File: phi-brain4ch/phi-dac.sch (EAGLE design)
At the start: 146 parts, among them IC1 PCM1792A, IC10 LM317, IC11 LM337, IC2 OPA1632D, IC3 OPA1632D, IC4 OPA1632D, IC6 OPA1632D, IC7 REG1117-5, IC8 ADP3301ARZ-3.3, IC9 MGJ2D121515SC, J1 CUI-RCJ-2123, J5 DC21P

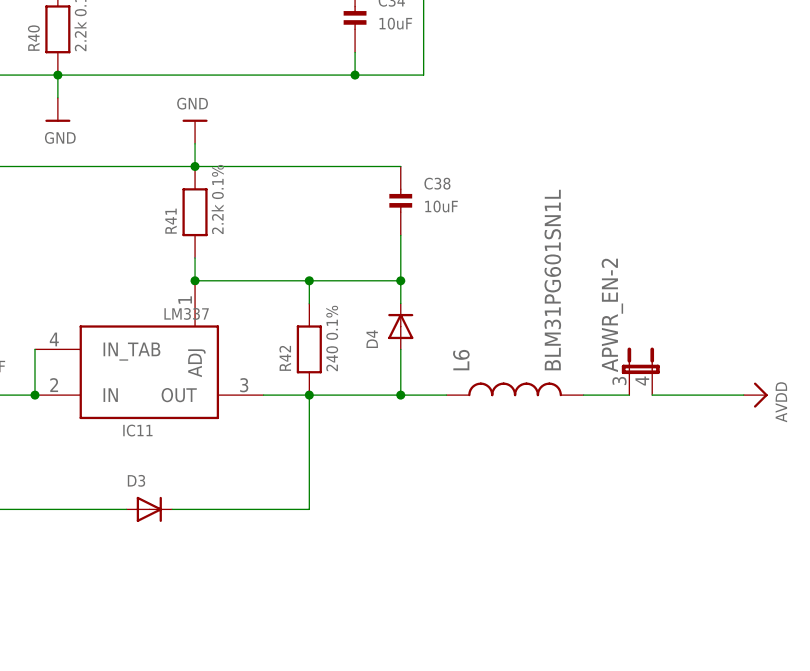
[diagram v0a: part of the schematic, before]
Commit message: wip
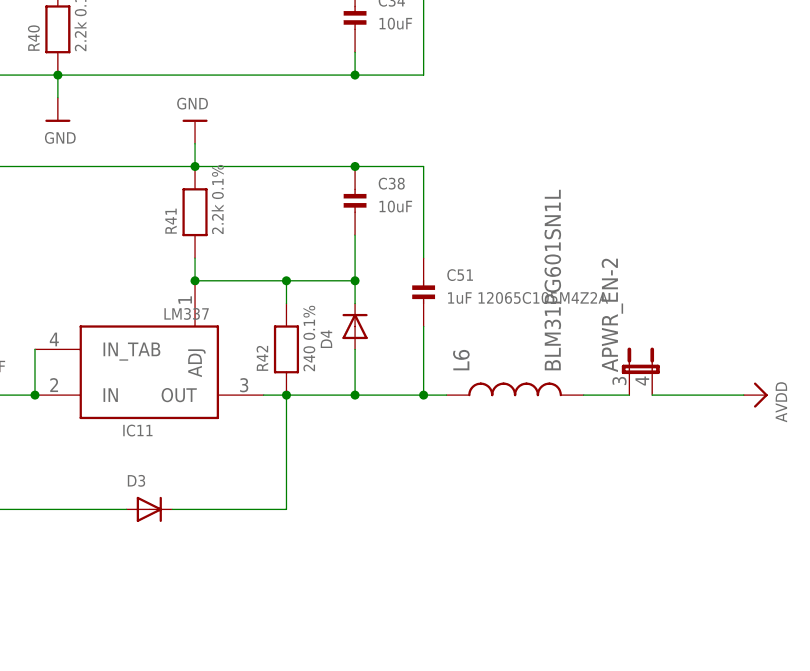
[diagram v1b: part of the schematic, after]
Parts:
- added C51: 1uF 12065C105M4Z2A, microbuilder:CAP_CERAMIC1206
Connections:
- net GND: now also C51.P$1
- net N$57: now also C51.P$2
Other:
- moved on the sheet: C38, D4, R42
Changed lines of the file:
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@@
 <part name="C49" library="microbuilder" deviceset="CAP_CERAMIC" device="0603" value="0.1u"/>
 <part name="C50" library="microbuilder" deviceset="CAP_CERAMIC" device="0603" value="0.1u"/>
+<part name="C51" library="microbuilder" deviceset="CAP_CERAMIC" device="1206" value="1uF 12065C105M4Z2A"/>
 </parts>
 <sheets>
@@
 <instance part="C37" gate="G$1" x="190.5" y="147.32"/>
 <instance part="R41" gate="G$1" x="218.44" y="165.1" rot="R90"/>
-<instance part="R42" gate="G$1" x="231.14" y="149.86" rot="R90"/>
+<instance part="R42" gate="G$1" x="228.6" y="149.86" rot="R90"/>
 <instance part="U$29" gate="G$1" x="218.44" y="175.26" rot="R180"/>
-<instance part="C38" gate="G$1" x="241.3" y="165.1"/>
-<instance part="D4" gate="G$1" x="241.3" y="152.4" rot="R90"/>
+<instance part="C38" gate="G$1" x="236.22" y="165.1"/>
+<instance part="D4" gate="G$1" x="236.22" y="152.4" rot="R90"/>
 <instance part="L6" gate="G$1" x="254" y="144.78" rot="R90"/>
 <instance part="U$30" gate="G$1" x="281.94" y="144.78" rot="R270"/>
@@
 <instance part="C49" gate="G$1" x="149.86" y="-22.86"/>
 <instance part="C50" gate="G$1" x="149.86" y="-12.7"/>
+<instance part="C51" gate="G$1" x="243.84" y="154.94"/>
 </instances>
 <busses>
@@
 <junction x="218.44" y="170.18"/>
 <pinref part="C38" gate="G$1" pin="P$1"/>
-<wire x1="218.44" y1="170.18" x2="241.3" y2="170.18" width="0.1524" layer="91"/>
+<wire x1="218.44" y1="170.18" x2="236.22" y2="170.18" width="0.1524" layer="91"/>
+<pinref part="C51" gate="G$1" pin="P$1"/>
+<wire x1="236.22" y1="170.18" x2="243.84" y2="170.18" width="0.1524" layer="91"/>
+<wire x1="243.84" y1="170.18" x2="243.84" y2="160.02" width="0.1524" layer="91"/>
+<junction x="236.22" y="170.18"/>
 </segment>
 <segment>
@@
 <pinref part="D3" gate="G$1" pin="C"/>
 <pinref part="R42" gate="G$1" pin="1"/>
-<wire x1="215.9" y1="132.08" x2="231.14" y2="132.08" width="0.1524" layer="91"/>
-<wire x1="231.14" y1="132.08" x2="231.14" y2="144.78" width="0.1524" layer="91"/>
+<wire x1="215.9" y1="132.08" x2="228.6" y2="132.08" width="0.1524" layer="91"/>
+<wire x1="228.6" y1="132.08" x2="228.6" y2="144.78" width="0.1524" layer="91"/>
 <pinref part="IC11" gate="G$1" pin="OUT"/>
-<wire x1="231.14" y1="144.78" x2="226.06" y2="144.78" width="0.1524" layer="91"/>
-<junction x="231.14" y="144.78"/>
-<wire x1="231.14" y1="144.78" x2="241.3" y2="144.78" width="0.1524" layer="91"/>
-<wire x1="241.3" y1="144.78" x2="241.3" y2="149.86" width="0.1524" layer="91"/>
+<wire x1="228.6" y1="144.78" x2="226.06" y2="144.78" width="0.1524" layer="91"/>
+<junction x="228.6" y="144.78"/>
+<wire x1="228.6" y1="144.78" x2="236.22" y2="144.78" width="0.1524" layer="91"/>
+<wire x1="236.22" y1="144.78" x2="236.22" y2="149.86" width="0.1524" layer="91"/>
 <pinref part="D4" gate="G$1" pin="A"/>
 <pinref part="L6" gate="G$1" pin="1"/>
-<wire x1="246.38" y1="144.78" x2="241.3" y2="144.78" width="0.1524" layer="91"/>
-<junction x="241.3" y="144.78"/>
+<wire x1="246.38" y1="144.78" x2="243.84" y2="144.78" width="0.1524" layer="91"/>
+<junction x="236.22" y="144.78"/>
+<junction x="243.84" y="144.78"/>
+<wire x1="243.84" y1="144.78" x2="236.22" y2="144.78" width="0.1524" layer="91"/>
+<pinref part="C51" gate="G$1" pin="P$2"/>
+<wire x1="243.84" y1="152.4" x2="243.84" y2="144.78" width="0.1524" layer="91"/>
 </segment>
 </net>
@@
 <wire x1="218.44" y1="157.48" x2="218.44" y2="160.02" width="0.1524" layer="91"/>
 <pinref part="R42" gate="G$1" pin="2"/>
-<wire x1="231.14" y1="154.94" x2="231.14" y2="157.48" width="0.1524" layer="91"/>
-<wire x1="231.14" y1="157.48" x2="218.44" y2="157.48" width="0.1524" layer="91"/>
+<wire x1="228.6" y1="154.94" x2="228.6" y2="157.48" width="0.1524" layer="91"/>
+<wire x1="228.6" y1="157.48" x2="218.44" y2="157.48" width="0.1524" layer="91"/>
 <junction x="218.44" y="157.48"/>
-<wire x1="231.14" y1="157.48" x2="241.3" y2="157.48" width="0.1524" layer="91"/>
-<wire x1="241.3" y1="157.48" x2="241.3" y2="154.94" width="0.1524" layer="91"/>
+<wire x1="228.6" y1="157.48" x2="236.22" y2="157.48" width="0.1524" layer="91"/>
+<wire x1="236.22" y1="157.48" x2="236.22" y2="154.94" width="0.1524" layer="91"/>
 <pinref part="C38" gate="G$1" pin="P$2"/>
-<wire x1="241.3" y1="157.48" x2="241.3" y2="162.56" width="0.1524" layer="91"/>
-<junction x="241.3" y="157.48"/>
+<wire x1="236.22" y1="157.48" x2="236.22" y2="162.56" width="0.1524" layer="91"/>
+<junction x="236.22" y="157.48"/>
 <pinref part="D4" gate="G$1" pin="C"/>
-<junction x="231.14" y="157.48"/>
-</segment>
-</net>
+<junction x="228.6" y="157.48"/>
+</segment>
+</net>
